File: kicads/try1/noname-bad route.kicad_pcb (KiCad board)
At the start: 2 copper layers, 35 parts, among them P2 GND, P3 CONN_01X08, P4 A2 A3 A4 A5 A6, P5 Mutual, P6 CONN_01X08, SW1 SW_PUSH, SW2 SW_PUSH, SW3 SW_PUSH, SW4 SW_PUSH, U2 CD74HCT4067, U3 CD74HCT4067

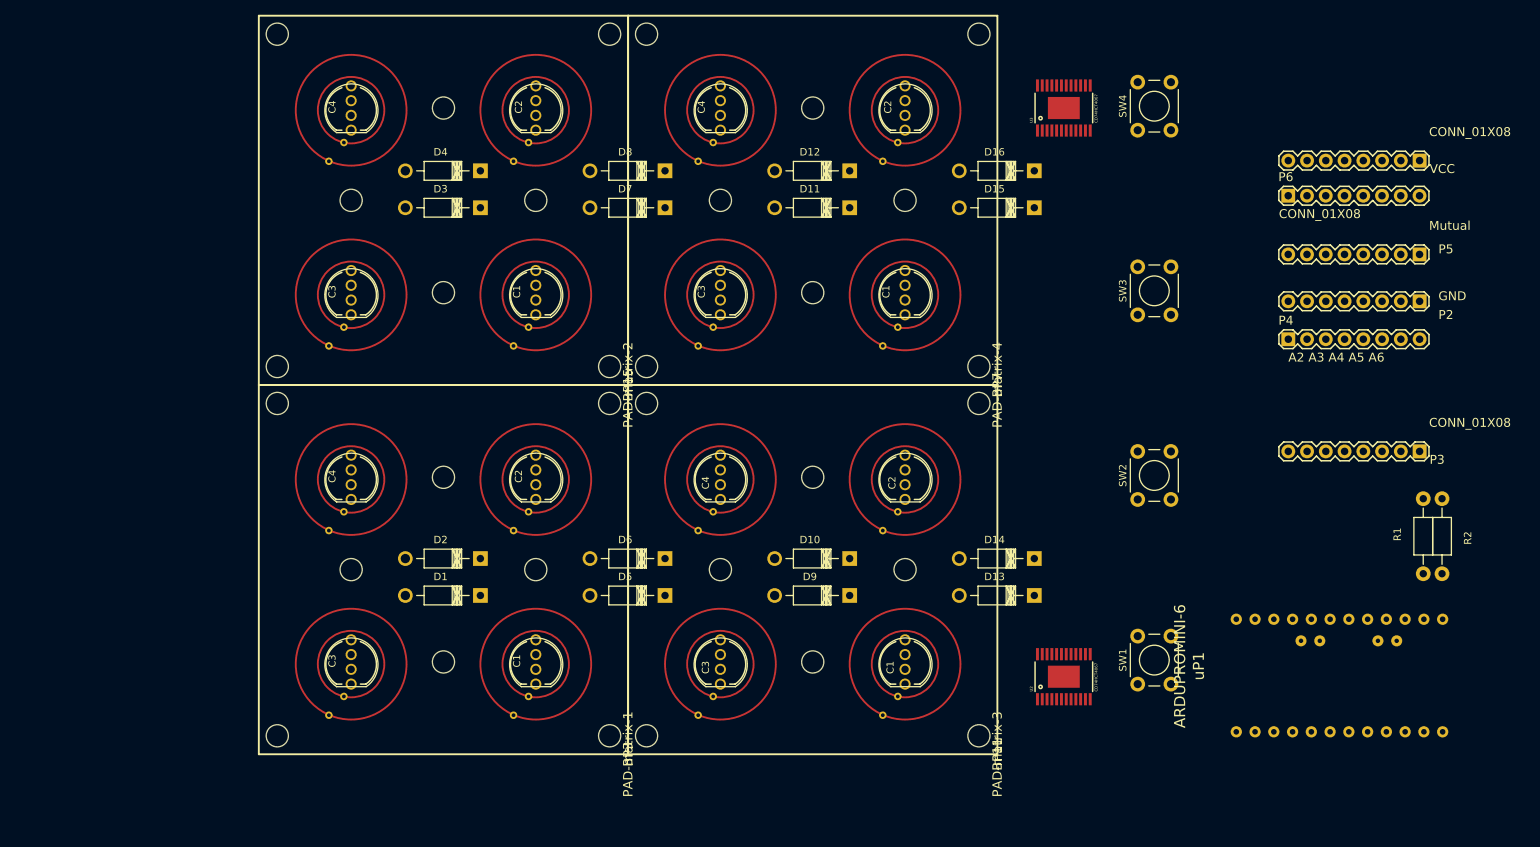
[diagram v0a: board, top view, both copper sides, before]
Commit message: forward with the pcb design
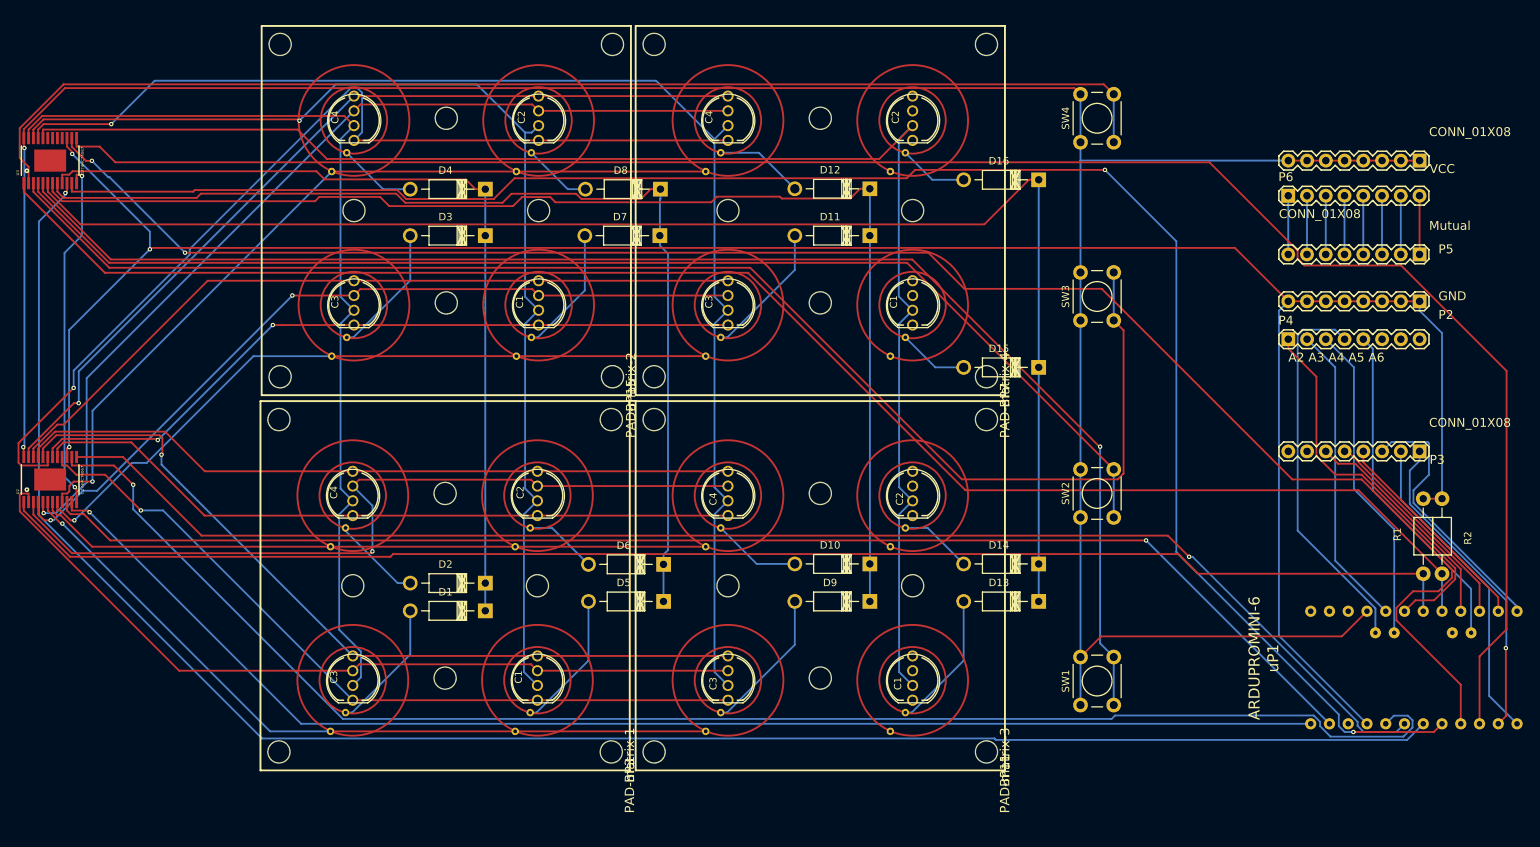
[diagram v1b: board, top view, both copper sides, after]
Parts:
- moved U2 139.8 mm to (31.8, 114.3)
- moved U3 137.4 mm to (31.8, 71.1)
- moved D15 21.6 mm to (165.6, 99.1)
- moved uP1 10.1 mm to (196.1, 149.9)
- moved SW1 8.25 mm to (171.3, 144.8)
- moved SW2 8.12 mm to (171.3, 119.4)
- moved SW4 7.92 mm to (171.3, 68.6)
- moved SW3 7.78 mm to (171.3, 92.8)
- moved D11 4.66 mm to (142.7, 81.3)
- moved D7 3.84 mm to (114.3, 81.3)
- moved D3 3.84 mm to (90.7, 81.3)
- moved D12 3.66 mm to (142.7, 74.9)
- moved D2 3.39 mm to (90.7, 128.3)
- moved D9 2.85 mm to (142.7, 130.8)
- moved D10 2.83 mm to (142.7, 125.7)
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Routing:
- net /VCC: track 0.00 -> 360.2 mm, vias 0 -> 2
- net GNDREF: track 0.00 -> 320.8 mm, vias 0 -> 3
- net /PD7: track 0.00 -> 257.3 mm
- net /PD4: track 0.00 -> 247.5 mm, vias 0 -> 1
- net /PD5: track 0.00 -> 246.5 mm, vias 0 -> 2
- net /PD6: track 0.00 -> 241.4 mm, vias 0 -> 2
- net /A0: track 0.00 -> 219.7 mm
- net /PD2: track 0.00 -> 206.4 mm, vias 0 -> 1
- net /MUXBG11: track 0.00 -> 202.8 mm
- net /A1: track 0.00 -> 199.6 mm
- net /MUXBS3: track 0.00 -> 196.8 mm
- net /PD3: track 0.00 -> 196.0 mm, vias 0 -> 1
- net /MUXBS4: track 0.00 -> 194.3 mm, vias 0 -> 1
- net /MUXBS6: track 0.00 -> 193.0 mm
- net /PD0: track 0.00 -> 184.0 mm, vias 0 -> 1
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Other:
- net class Default: clearance 0.4 -> 0.2; trace_width 0.4 -> 0.25
- net class seeed removed
- rule trace_clearance: 0.4 -> 0.2
